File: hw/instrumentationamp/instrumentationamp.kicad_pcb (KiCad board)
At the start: 2 copper layers, 10 x 10 mm, 18 parts, among them U1 Opamp_Quad_Generic

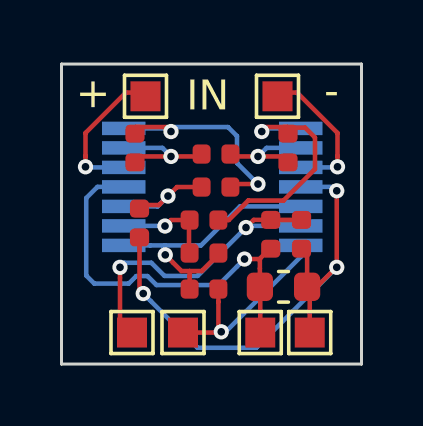
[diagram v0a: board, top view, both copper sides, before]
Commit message: proper Viset and final stage on instrumentation amp
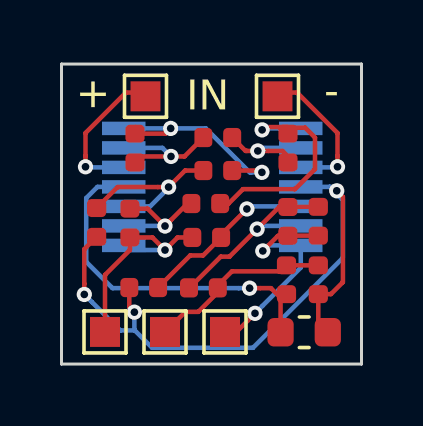
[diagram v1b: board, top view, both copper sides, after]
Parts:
- removed TP5, TP6: Test_Point, TestPoint:TestPoint_Pad_1.0x1.0mm
- added C2: 10n, Capacitor_SMD:C_0402_1005Metric, F.Cu at (111.9, 73.5)
- added R11: 1K, Resistor_SMD:R_0402_1005Metric, F.Cu at (108.2, 74.1)
- added R12: 250k, Resistor_SMD:R_0402_1005Metric, F.Cu at (106.1, 75.8)
- added R13: 250k, Resistor_SMD:R_0402_1005Metric, F.Cu at (110.9, 73.5)
- added TP4: Test_Point, TestPoint:TestPoint_Pad_1.0x1.0mm, F.Cu at (104.8, 77.2)
- R1: value 2K -> 1K
- R10: value DNI -> 1k
- R2, R3: value 4K02 -> 2K
- R9: value 100K -> 1M
- U1: value Opamp_Quad_Generic -> TLV274
- moved R7 2.66 mm to (105.6, 73.6), turned to 90 degrees
- moved C1 1.66 mm to (111.4, 77.2)
- moved R9 1.62 mm to (111.9, 75.5)
- moved R8 1.60 mm to (110.8, 75.5)
- moved R6 1.43 mm to (104.5, 73.6)
- moved TP7 1.40 mm to (108.8, 77.2)
- moved TP3 1.10 mm to (106.8, 77.2)
- moved R5 0.55 mm to (108.6, 71.8)
- moved R1 0.55 mm to (108.6, 70.8)
- moved R4 0.55 mm to (108.2, 73.0)
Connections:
- net Net-(TP1-Pad1) renamed /Vin-
- net Net-(TP2-Pad1) renamed /Vin+
- R10 pad 1: /vout -> /Viset
- R10 pad 2: Net-(R10-Pad2) -> Net-(C2-Pad2)
- R7 pad 1: Net-(R10-Pad2) -> /Vimeas
- R8 pad 1: Net-(R8-Pad1) -> /Viset
- R9 pad 2: Net-(R8-Pad1) -> /Viset
- TP3 pad 1: Net-(R8-Pad1) -> /Viset
- U1 pad 1: Net-(R10-Pad2) -> /Vimeas
- U1 pad 12: Net-(R10-Pad2) -> Net-(R11-Pad1)
- U1 pad 13: Net-(R8-Pad1) -> Net-(C2-Pad2)
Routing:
- net Net-(R8-Pad1): track 11.2 -> 0.00 mm, vias 2 -> 0
- net Net-(R10-Pad2): track 9.66 -> 0.00 mm, vias 1 -> 0
- net /Vimeas: track 0.00 -> 7.54 mm, vias 0 -> 1
- net Net-(C2-Pad2): track 0.00 -> 6.93 mm, vias 0 -> 1
- net /Viset: track 0.00 -> 6.18 mm
- net Net-(R11-Pad1): track 0.00 -> 5.93 mm, vias 0 -> 1
- net GND: track 18.7 -> 23.6 mm
- net Net-(R5-Pad1): track 3.91 -> 5.86 mm
- net VCC: track 13.7 -> 11.8 mm
- net Net-(R4-Pad1): track 3.36 -> 4.26 mm
- net /vout: track 6.81 -> 7.67 mm, vias 1 -> 2
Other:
- board text added: "inst.amp. v2"
- board text removed: "inst.amp. v1"
